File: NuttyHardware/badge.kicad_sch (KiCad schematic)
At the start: 119 parts, among them J1 RGB_OUT, J2 CC_MODULE, J3 Micro_SD_Card_Det, J4 Expose_GPIOs, J5 I2C_Pins, J6 Power_Pins, J7 Expose_SDPins, Q1 MMBT3904, Q2 MMBT3904, Q3 IRF9321PbF, Q4 MMBT3904, Q5 MMBT3904, Q6 MMBT3904, Q7 MMBT3904, SW1 BTN_UP, SW10 SW_DPDT_x2, SW2 BTN_RIGHT, SW3 BTN_SELECT, SW4 BTN_DOWN, SW5 BTN_A, SW6 BTN_START, SW7 BTN_LEFT, SW8 BTN_B, SW9 BTN_USRDEF, U1 PCF8574T, U2 LuatOS-ESP32S3-Module, U3 AMS1117-3.3, U4 IRM-3638T, U5 GM12864T-5D_SPILCD, U6 TPS63001

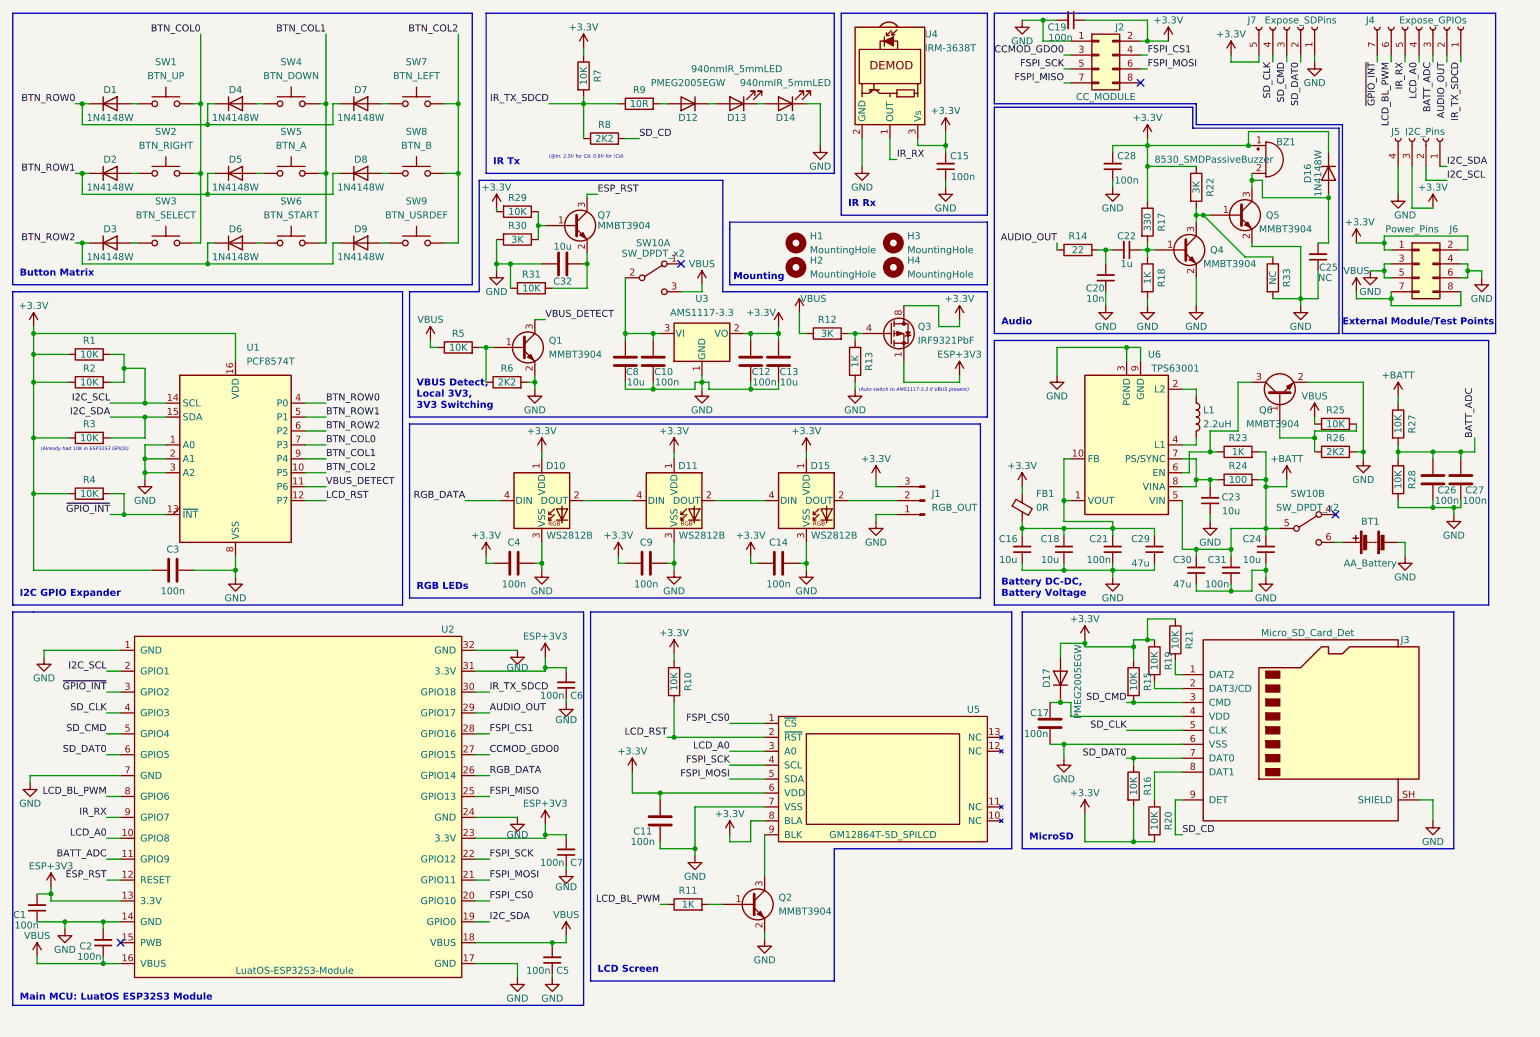
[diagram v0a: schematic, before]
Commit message: [HARDWARE] NuttyBadge Revision B
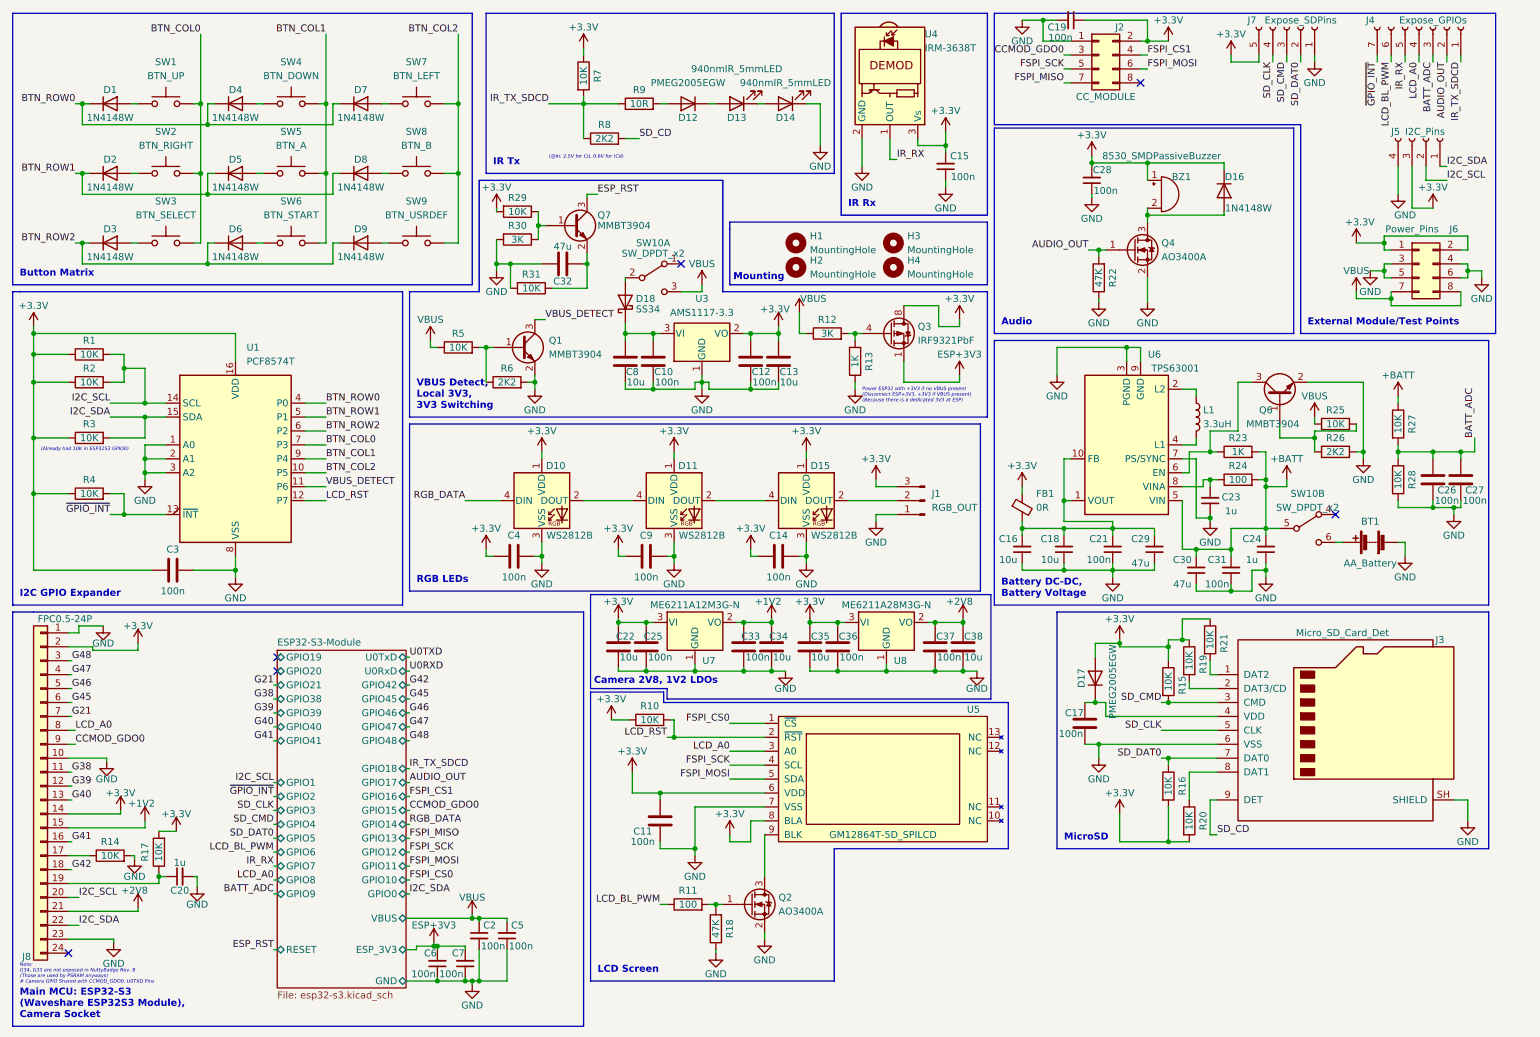
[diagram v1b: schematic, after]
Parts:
- removed C1: 100n, Capacitor_SMD:C_1206_3216Metric_Pad1.33x1.80mm_HandSolder, symbol Device:C_Small
- removed C22: 1u, Capacitor_SMD:C_1206_3216Metric_Pad1.33x1.80mm_HandSolder, symbol Device:C_Small
- removed C25: NC, Capacitor_SMD:C_1206_3216Metric_Pad1.33x1.80mm_HandSolder, symbol Device:C_Small
- removed Q2, Q4, Q5: MMBT3904, Package_TO_SOT_SMD:SOT-23, symbol Transistor_BJT:MMBT3904
- removed R33: NC, Resistor_SMD:R_1206_3216Metric_Pad1.30x1.75mm_HandSolder, symbol Device:R
- removed U2: LuatOS-ESP32S3-Module, Custom:Module_ESP32S3_LuatOS, symbol ESP32S3_Module:LuatOS-ESP32S3-Module
- added C22, C34, C35, C38: 10u, Capacitor_SMD:C_1206_3216Metric_Pad1.33x1.80mm_HandSolder, symbol Device:C
- added C25, C33, C36, C37: 100n, Capacitor_SMD:C_1206_3216Metric_Pad1.33x1.80mm_HandSolder, symbol Device:C
- added D18: SS34, Custom:D_SMA_Handsoldering-BigDiodeSilkscreen, symbol Diode:1N5822
- added J8: FPC0.5-24P, Connector_FFC-FPC:Jushuo_AFC07-S24FCA-00_1x24-1MP_P0.50_Horizontal, symbol Connector_Generic:Conn_01x24
- added Q2, Q4: AO3400A, Package_TO_SOT_SMD:SOT-23, symbol Transistor_FET:AO3400A
- added U7: ME6211A12M3G-N, Package_TO_SOT_SMD:SOT-23-3, symbol LDO_Regulators:ME6211A12M3G-N
- added U8: ME6211A28M3G-N, Package_TO_SOT_SMD:SOT-23-3, symbol LDO_Regulators:ME6211A28M3G-N
- C20: value 10n -> 1u
- C23, C24: value 10u -> 1u
- C32: value 10u -> 47u
- L1: value 2.2uH -> 3.3uH
- R11: value 1K -> 100
- R14: value 22 -> 10K
- R17: value 330 -> 10K
- R18: value 1K -> 47K
- R22: value 3K -> 47K
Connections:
- net +3.3V: now also R17.2, C22.2, C25.2, C35.2, C36.2, J8.14 (Pin_14), J8.2 (Pin_2), U7.3 (VI), U8.3 (VI); no longer R17.1, R22.1
- net AUDIO_OUT: now also R22.2, Q4.1 (G); no longer R14.1
- net CCMOD_GDO0: now also J8.9 (Pin_9)
- net GND: now also C20.2, R14.2, R18.1, R22.1, U6.7 (PS/SYNC), C22.1, C25.1, C33.1, C34.1, C35.1, C36.1, C37.1, C38.1, J8.1 (Pin_1), J8.10 (Pin_10), J8.23 (Pin_23), Q2.2 (S), Q4.2 (S), U7.1 (GND), U8.1 (GND); no longer C20.1, R18.2
- net I2C_SCL: now also J8.20 (Pin_20)
- net I2C_SDA: now also J8.22 (Pin_22)
- net LCD_A0: now also J8.8 (Pin_8)
- net at C10.2, C8.2, U3.3 (VI): now also D18.1 (K); no longer SW10.2 (B)
- net at BZ1.2 (+), D16.2 (A): now also Q4.3 (D)
- net at C23.2, R24.1, U6.8 (VINA): no longer U6.7 (PS/SYNC)
- net at U5.9 (BLK): now also Q2.3 (D)
- net at R11.2: now also R18.2, Q2.1 (G)
- new net: J8.17 (Pin_17), R14.1
- new net: C20.1, J8.19 (Pin_19), R17.1
- new net: D18.2 (A), SW10.2 (B)
- new net +1V2: C33.2, C34.2, J8.15 (Pin_15), U7.2 (VO)
- new net +2V8: C37.2, C38.2, J8.21 (Pin_21), U8.2 (VO)
- new net G21: J8.7 (Pin_7)
- new net G38: J8.11 (Pin_11)
- new net G39: J8.12 (Pin_12)
- new net G40: J8.13 (Pin_13)
- new net G41: J8.16 (Pin_16)
- new net G42: J8.18 (Pin_18)
- new net G45: J8.6 (Pin_6)
- new net G46: J8.5 (Pin_5)
- new net G47: J8.4 (Pin_4)
- new net G48: J8.3 (Pin_3)
- no-connect marks 4 -> 6
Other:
- added sheet ESP32-S3-Module (esp32-s3.kicad_sch)
- note added: "Camera 2V8, 1V2 LDOs"
- note added: "Main MCU: ESP32-S3 (Waveshare ESP32S3 Module), Camera Socket"
- note added: "Note: G34, G33 are not exposed in NuttyBadge Rev. B (Those are used by PSRAM anyways) # Camera GPIO Shared with CCMOD_GDO0, U0TXD Pins"
- note added: "Power ESP32 with +3V3 if no VBUS present (Disconnect ESP+3V3, +3V3 if VBUS present) (Because there is a dedicated 3V3 at ESP)"
- note removed: "(Auto switch to AMS1117-3.3 if VBUS present)"
- note removed: "Main MCU: LuatOS ESP32S3 Module"
- title: NuttyBadge Rev. A -> NuttyBadge Rev. B
- moved on the sheet: BZ1, C14, C17, C2, C28, C4, C5, C9, D16, D17, J3, R10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
